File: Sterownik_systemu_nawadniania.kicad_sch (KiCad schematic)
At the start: 44 parts

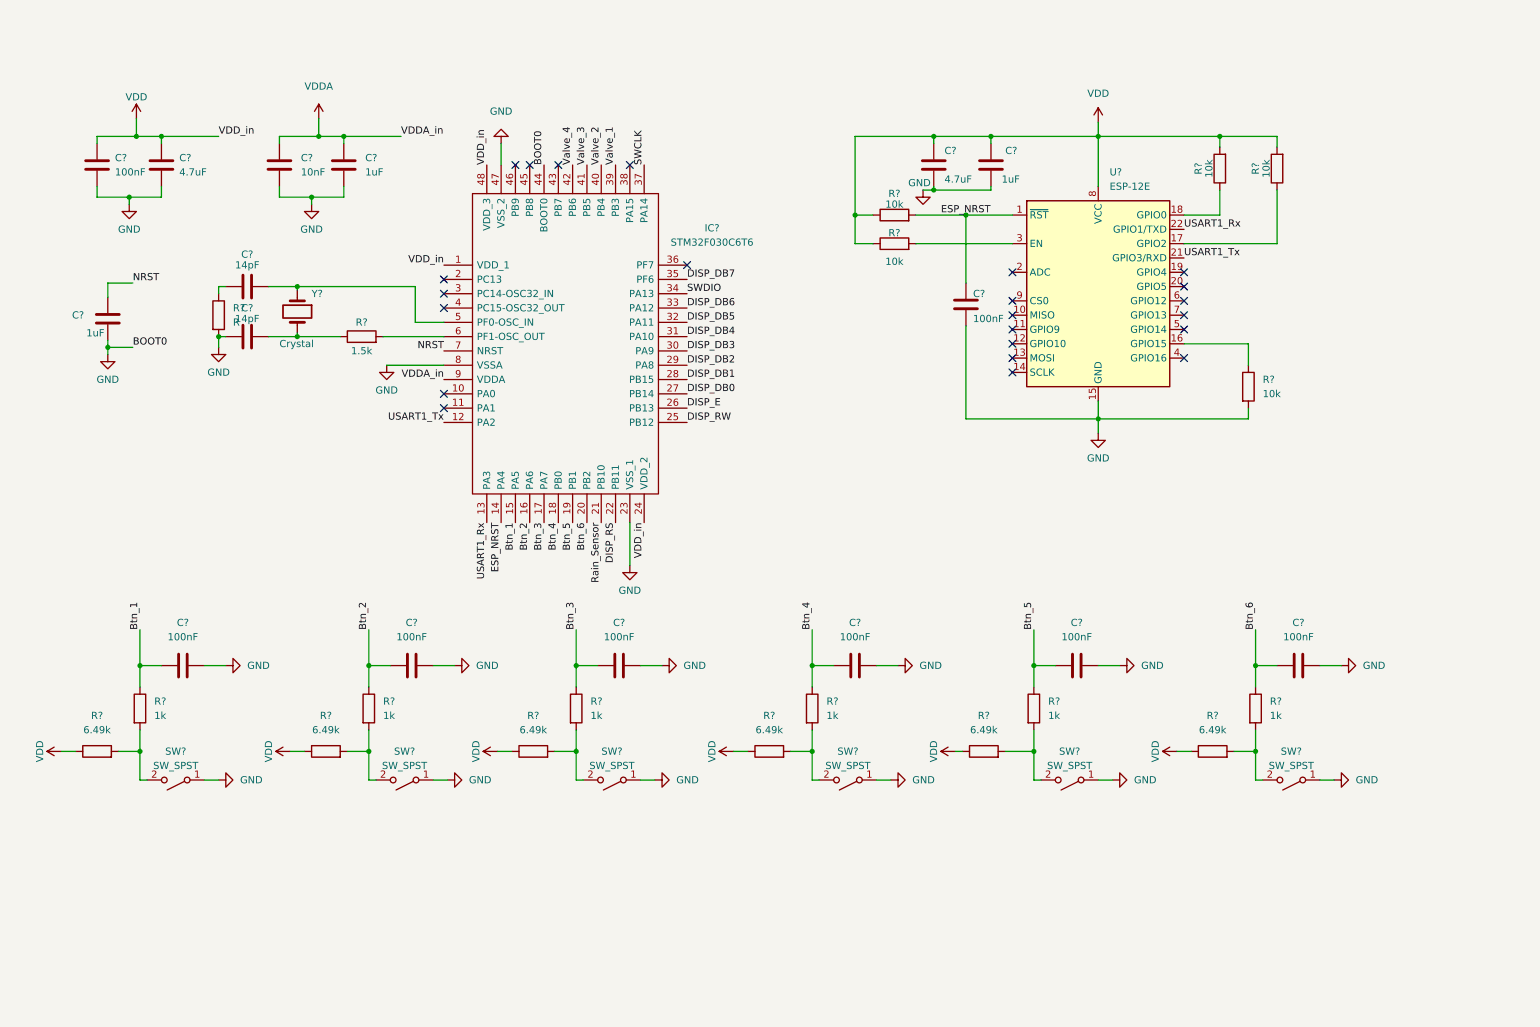
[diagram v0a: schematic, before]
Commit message: power unit
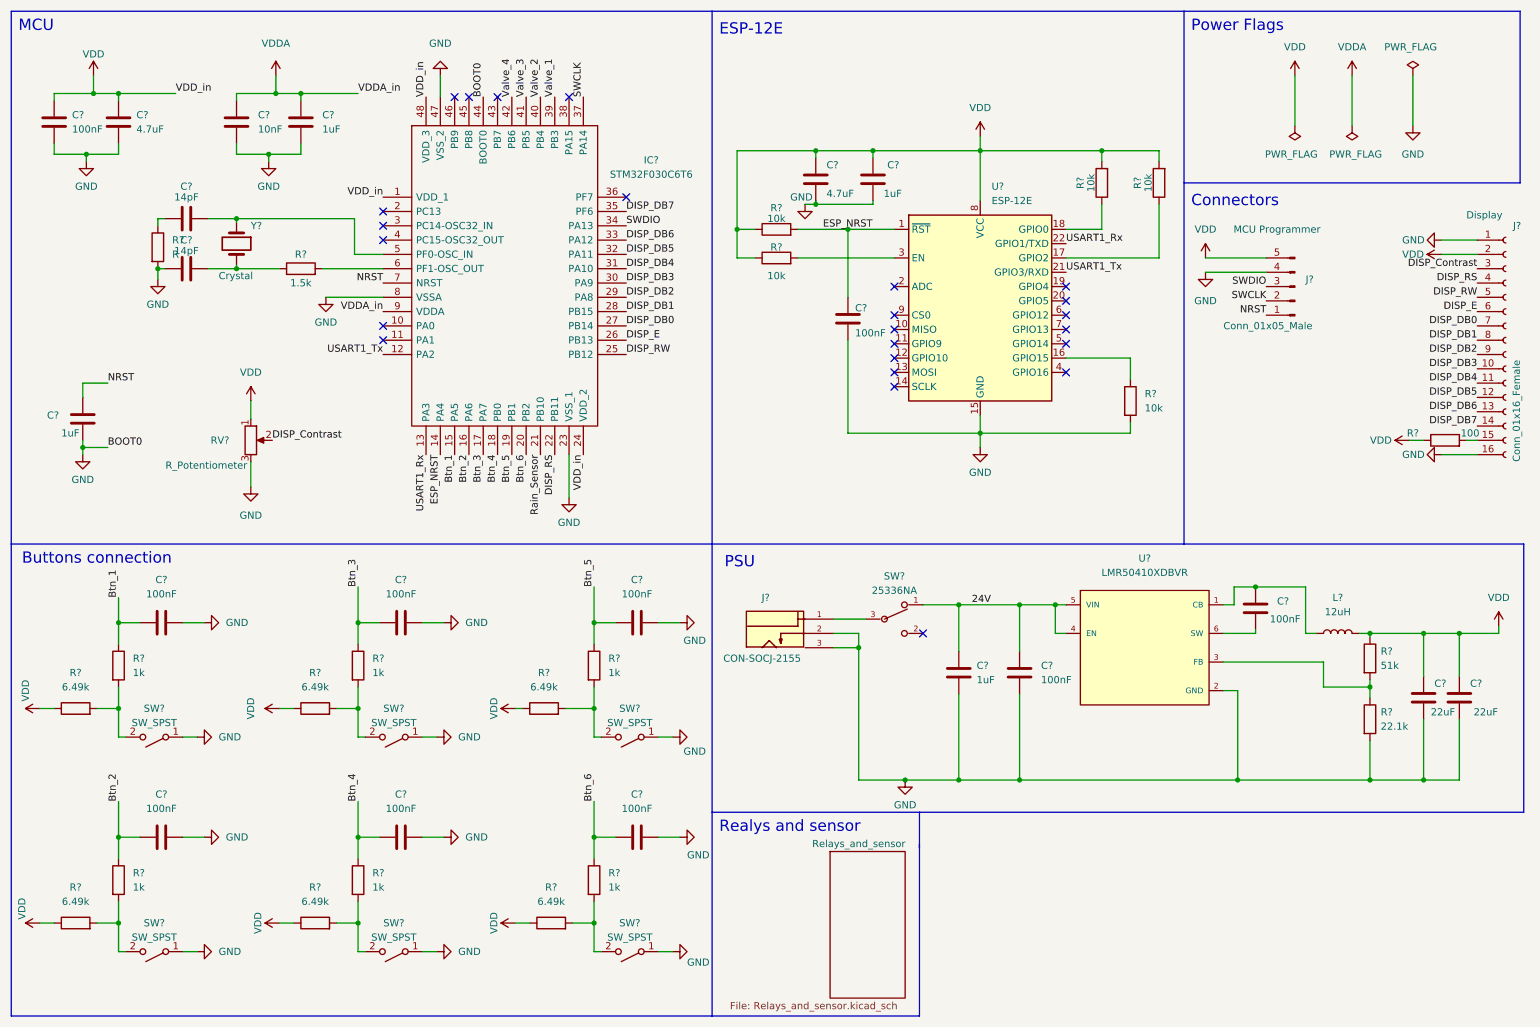
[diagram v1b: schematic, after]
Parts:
- added C?: 1uF, symbol Device:C
- added C? (x2): 22uF, symbol Device:C
- added C? (x2): 100nF, symbol Device:C
- added J?: Conn_01x05_Male, symbol Connector:Conn_01x05_Male
- added J?: CON-SOCJ-2155, GRAVITECH_CON-SOCJ-2155, symbol CON-SOCJ-2155:CON-SOCJ-2155
- added J?: Conn_01x16_Female, symbol Connector:Conn_01x16_Female
- added L?: 12uH, symbol Device:L
- added R?: 100, symbol Device:R
- added R?: 51k, symbol Device:R
- added R?: 22.1k, symbol Device:R
- added RV?: R_Potentiometer, symbol Device:R_Potentiometer
- added SW?: 25336NA, Apem_Inc.-25336NA-*, symbol eec2:25336NA
- added U?: LMR50410XDBVR, Texas_Instruments-DBV0006A-0-0-*, symbol eec:LMR50410XDBVR
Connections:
- net DISP_DB0: now also J?.7 (Pin_7)
- net DISP_DB1: now also J?.8 (Pin_8)
- net DISP_DB2: now also J?.9 (Pin_9)
- net DISP_DB3: now also J?.10 (Pin_10)
- net DISP_DB4: now also J?.11 (Pin_11)
- net DISP_DB5: now also J?.12 (Pin_12)
- net DISP_DB6: now also J?.13 (Pin_13)
- net DISP_DB7: now also J?.14 (Pin_14)
- net DISP_E: now also J?.6 (Pin_6)
- net DISP_RS: now also J?.4 (Pin_4)
- net DISP_RW: now also J?.5 (Pin_5)
- net GND: now also C?.2, C?.2, C?.2, C?.2, J?.1 (Pin_1), J?.16 (Pin_16), J?.2, J?.3, J?.4 (Pin_4), R?.2, RV?.3, U?.2 (GND)
- net NRST: now also J?.1 (Pin_1)
- net SWCLK: now also J?.2 (Pin_2)
- net SWDIO: now also J?.3 (Pin_3)
- net VDD: now also C?.1, C?.1, J?.2 (Pin_2), J?.5 (Pin_5), L?.2, R?.1, R?.1, RV?.1
- new net: J?.15 (Pin_15), R?.2
- new net: C?.1, L?.1, U?.1 (CB)
- new net: R?.1, R?.2, U?.3 (FB)
- new net: C?.2, U?.6 (SW)
- new net: J?.1, SW?.3 (Common)
- new net 24V: C?.1, C?.1, SW?.1, U?.4 (EN), U?.5 (VIN)
- new net DISP_Contrast: J?.3 (Pin_3), RV?.2
- no-connect marks 23 -> 24
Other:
- added sheet Relays_and_sensor (Relays_and_sensor.kicad_sch)
- note added: "Buttons connection"
- note added: "Connectors"
- note added: "ESP-12E"
- note added: "MCU"
- note added: "PSU"
- note added: "Power Flags"
- note added: "Realys and sensor"
- moved on the sheet: C?, IC?, R?, SW?, U?, Y?
